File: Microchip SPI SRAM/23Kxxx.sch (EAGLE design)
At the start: 5 parts, among them IC2 23KP, Q1 BSS101

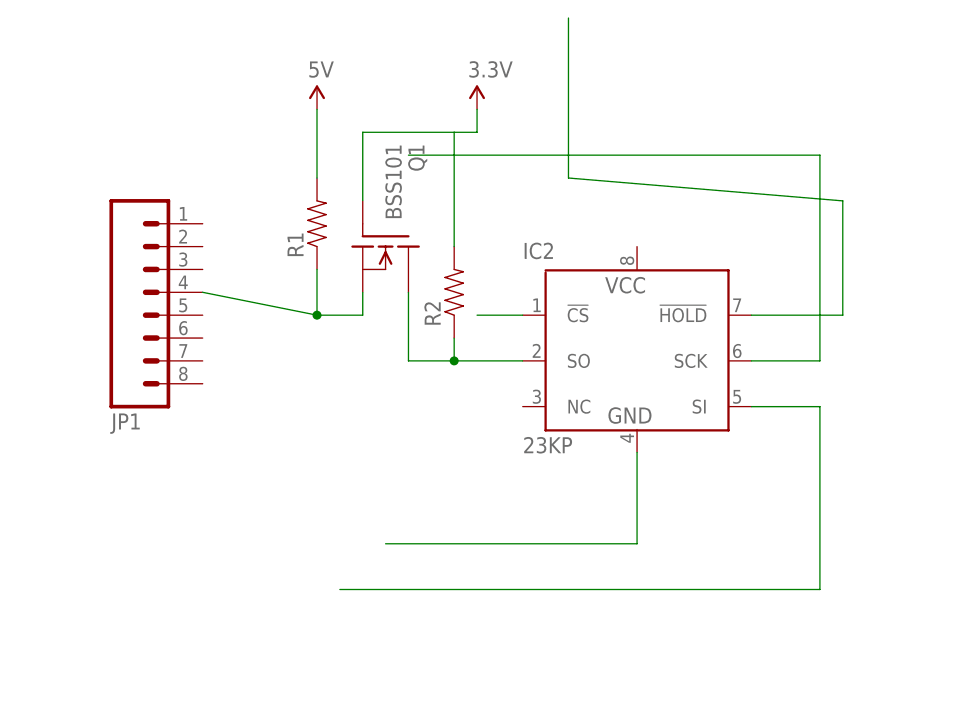
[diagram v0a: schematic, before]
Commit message: SRAM
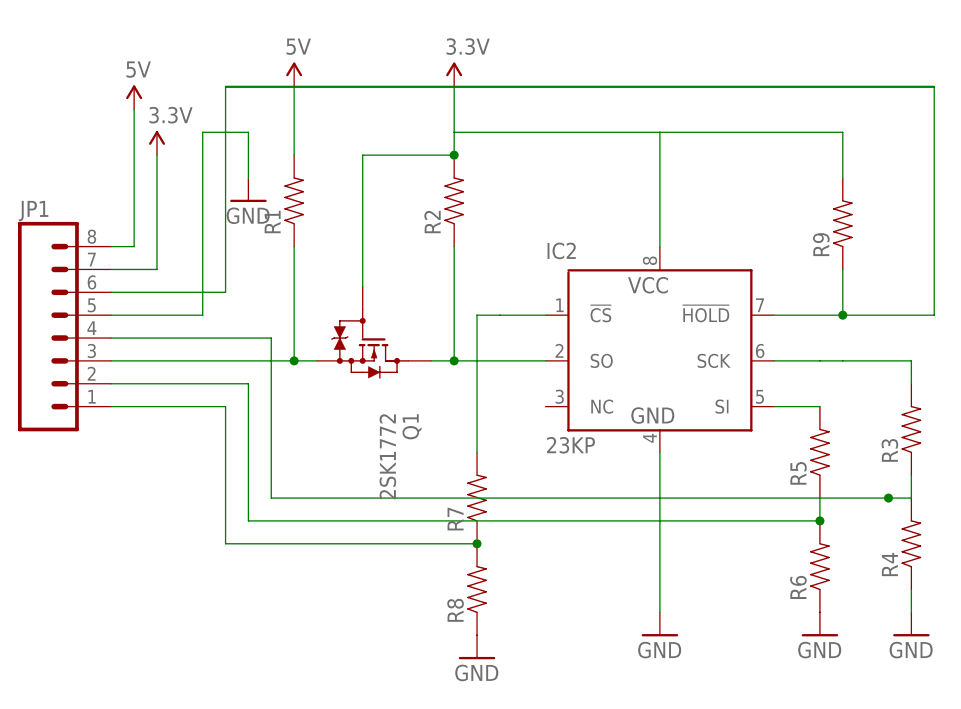
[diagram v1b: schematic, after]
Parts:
- added R3, R4, R5, R6, R7, R8, R9: (no value), My Library:RESISTORAXIAL-0.3
- Q1: value BSS101 -> 2SK1772; device transistor-fet:BSS101 -> My Library:2SK1772
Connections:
- removed net N$1: IC2.GND
- new net GND: IC2.GND, JP1.5, R4.1, R6.1, R8.1
- new net N$11: JP1.1, R7.1, R8.2
- new net N$8: JP1.2, R5.1, R6.2
- new net N$9: IC2.SI, R5.2
- net 3.3V: now also IC2.VCC, JP1.7, R9.2
- net 5V: now also JP1.8
- net N$2: now also JP1.3; no longer JP1.4
- net N$4: now also R7.2
- net N$5: now also JP1.6, R9.1
- net N$6: now also R3.2
- net N$7: now also JP1.4, R3.1, R4.2; no longer IC2.SI
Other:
- moved on the sheet: IC2, JP1, R1, R2
